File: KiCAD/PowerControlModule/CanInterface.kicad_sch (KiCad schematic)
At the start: 15 parts, among them J3 DF11-8DP-2DS, U7 MCP2515-xSO, U8 MCP2562-E-SN, U9 MCP1792x-5002xCB, Y1 8MHz

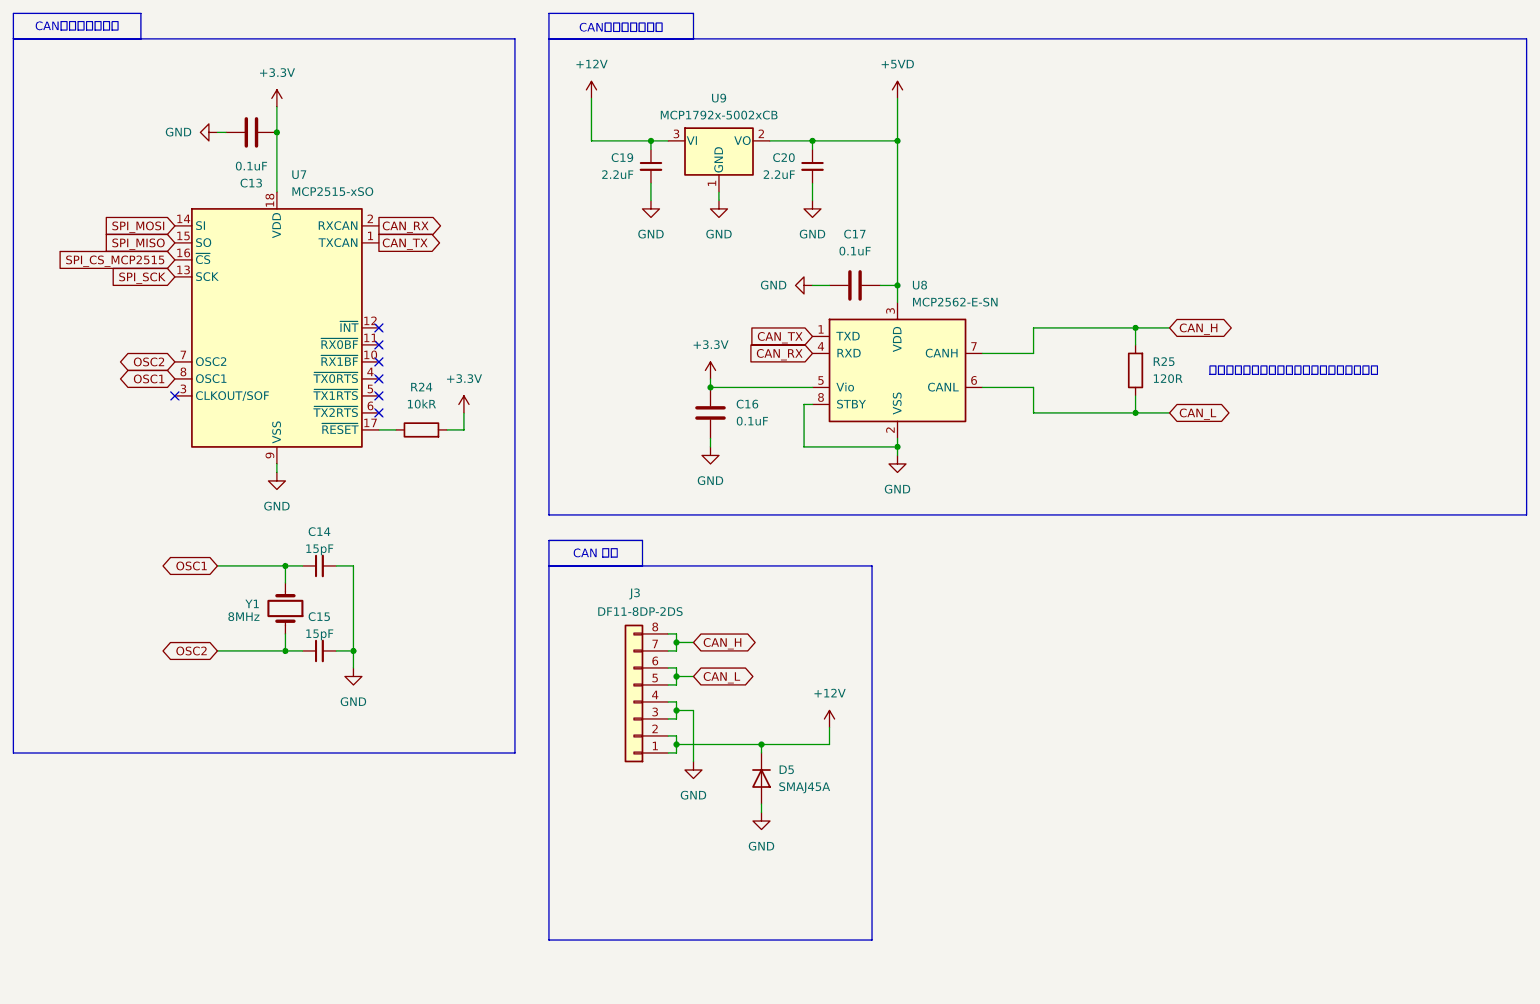
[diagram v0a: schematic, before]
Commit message: Build-4作成完了
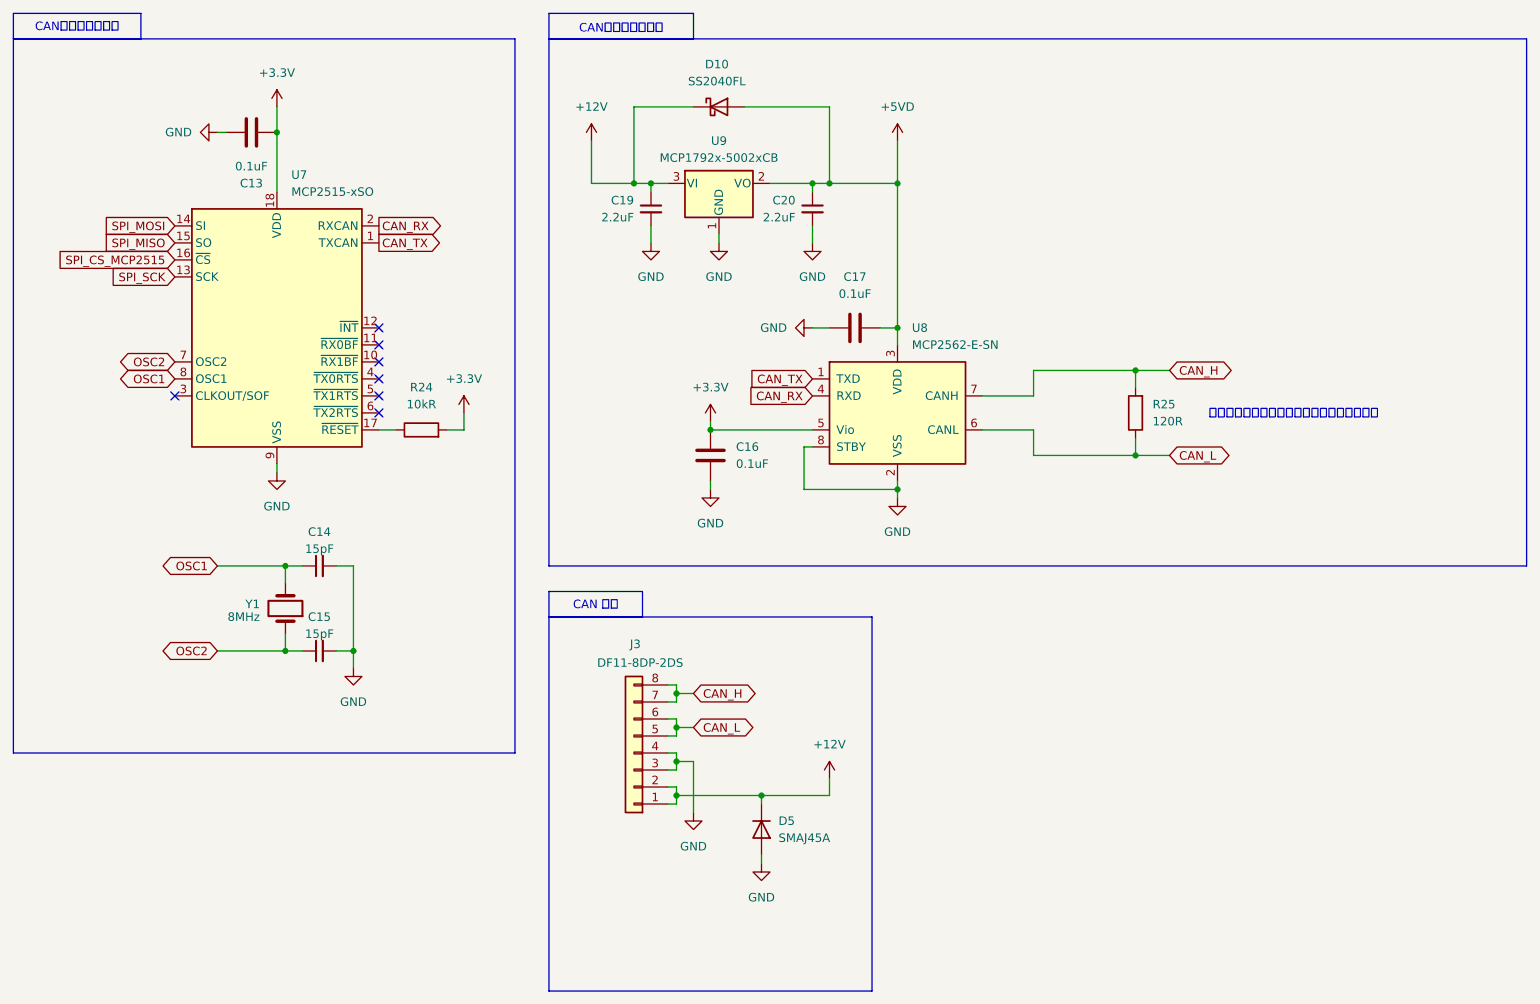
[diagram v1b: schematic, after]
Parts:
- added D10: SS2040FL, Diode_SMD:D_SOD-123F, symbol Device:D_Schottky
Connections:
- net +12V: now also D10.1 (K)
- net +5VD: now also D10.2 (A)
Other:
- moved on the sheet: C16, C17, C19, C20, D5, J3, R25, U8, U9
